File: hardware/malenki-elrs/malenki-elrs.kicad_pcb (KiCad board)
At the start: 4 copper layers, 19 x 32 mm, 64 parts, among them J1 Conn_01x02_Male-Connector, J2 PROG Header, J3 Weapons, J4 Conn_01x02_Male-Connector, J5 Conn_01x02_Male-Connector, J6 Conn_01x02_Male-Connector, U1 SPX3819M5-L-3-3, U3 SX1280IMLTRT, U4 DRV8837DSGR, U5 DRV8837DSGR, U6 DRV8837DSGR, U7 ESP32-S3FN8, Y1 ECS-400-10-37B2-CKY-TR, Y2 CRYSTAL 52MHz 10pF SMD

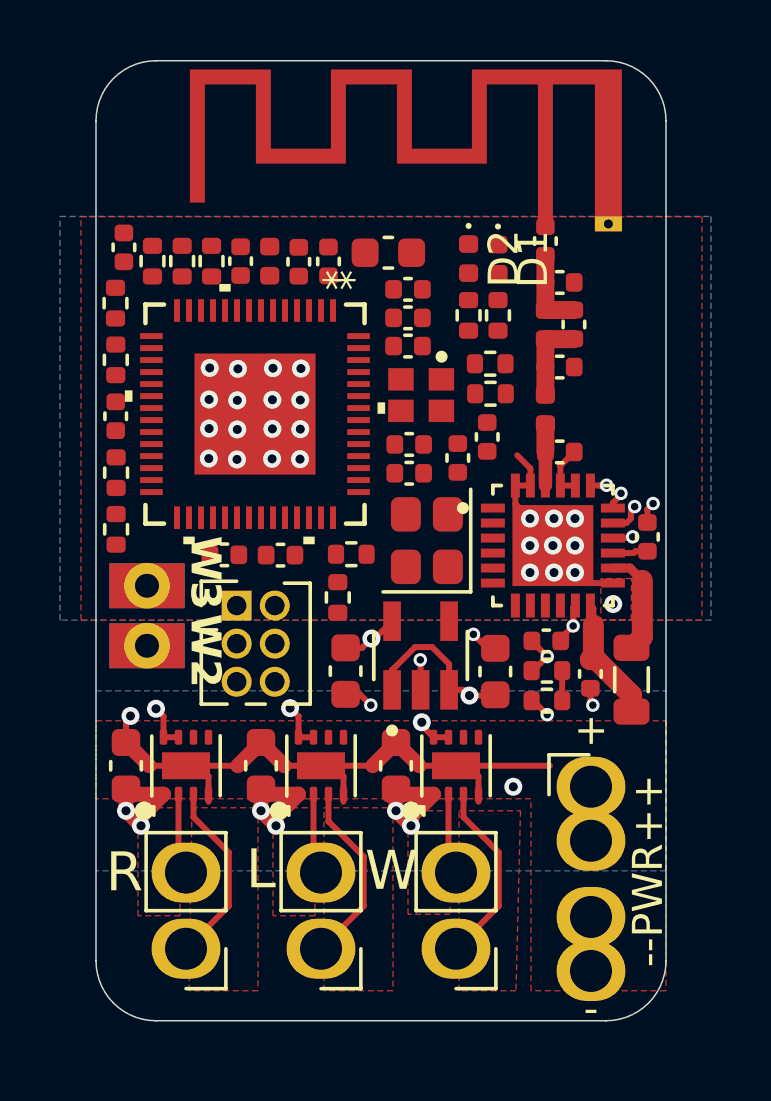
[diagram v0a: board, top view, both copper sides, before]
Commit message: Completed trace placement
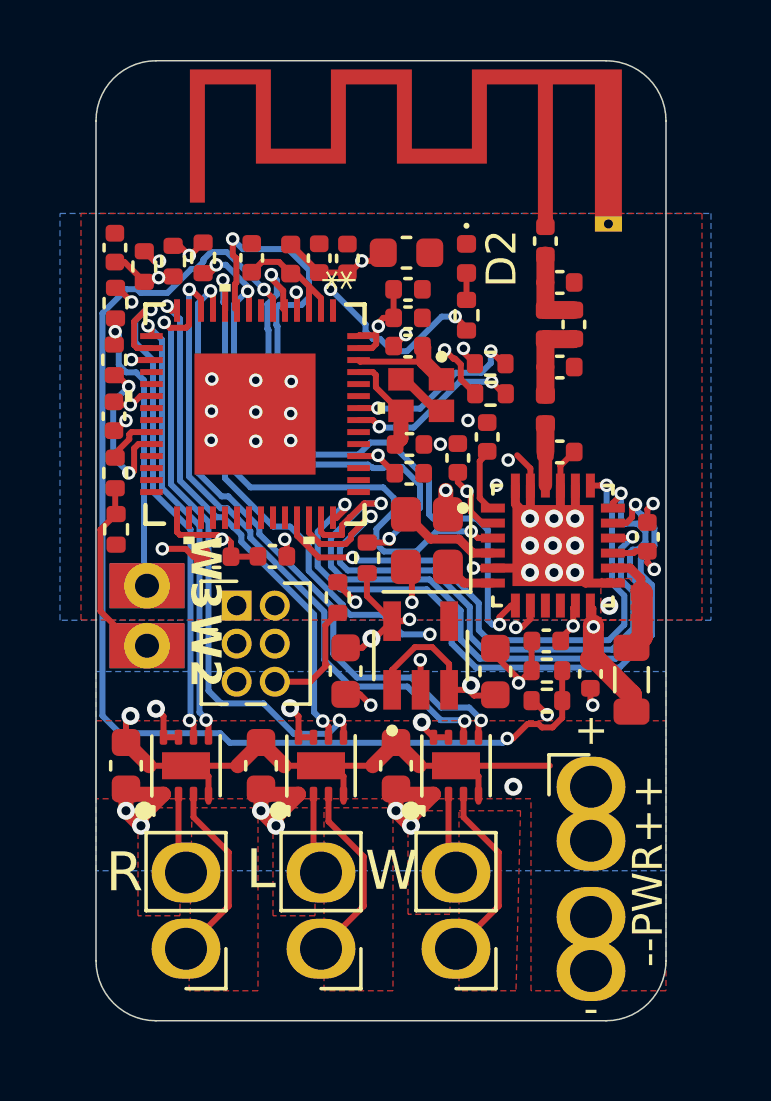
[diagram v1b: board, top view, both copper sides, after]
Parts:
- removed D1: LED Blue, LED_SMD:LED_0402_1005Metric
- removed R9: 470, Resistor_SMD:R_0402_1005Metric
- moved L4 0.70 mm to (94.5, 56.1)
- moved C12 0.69 mm to (95.4, 56.1), turned to 90 degrees
- moved C11 0.64 mm to (96.4, 56.1), turned to 90 degrees
- moved C14 0.60 mm to (98.3, 55.9)
- moved R13 0.54 mm to (97.0, 66.1), turned to -90 degrees
- moved C10 0.39 mm to (93.2, 56.1)
- moved R5 0.33 mm to (89.6, 56.4)
- moved R15 0.30 mm to (91.6, 56.1)
- moved R6 0.30 mm to (90.6, 56.2)
- moved C4 0.30 mm to (88.6, 55.7)
- moved C9 0.27 mm to (93.9, 66.0)
- moved C15 0.27 mm to (92.0, 66.0)
- moved D2 0.07 mm to (100.3, 56.1)
- moved R10 0.07 mm to (100.3, 58.0)
- moved C13 0.06 mm to (88.6, 61.4)
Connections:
- U7 pad 18: BLINKY -> unconnected-(U7-GPIO13-Pad18)
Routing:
- net VSENSE: track 1.00 -> 38.8 mm, vias 0 -> 2
- net BUSY: track 0.00 -> 25.8 mm, vias 0 -> 2
- net RADIO_SCK: track 0.55 -> 25.1 mm, vias 1 -> 2
- net RADIO_MOSI: track 1.12 -> 23.0 mm, vias 1 -> 2
- net DIO1: track 0.00 -> 21.6 mm, vias 0 -> 3
- net MOTOR1F: track 0.00 -> 21.5 mm, vias 0 -> 2
- net MOTOR1R: track 0.00 -> 21.3 mm, vias 0 -> 2
- net RADIO_NRESET: track 0.00 -> 20.8 mm, vias 0 -> 3
- net U0RXD: track 0.00 -> 20.5 mm, vias 0 -> 1
- net RADIO_MISO: track 0.68 -> 21.0 mm, vias 1 -> 2
- net MOTOR2F: track 0.00 -> 20.1 mm, vias 0 -> 2
- net Net-(U7-GPIO0): track 0.00 -> 19.7 mm, vias 0 -> 3
- net U0TXD: track 0.00 -> 19.2 mm, vias 0 -> 1
- net RADIO_NSS: track 0.54 -> 19.1 mm, vias 1 -> 2
- net VLOGIC: track 8.78 -> 27.1 mm, vias 5 -> 13
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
